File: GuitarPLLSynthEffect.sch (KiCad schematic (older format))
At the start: 26 parts

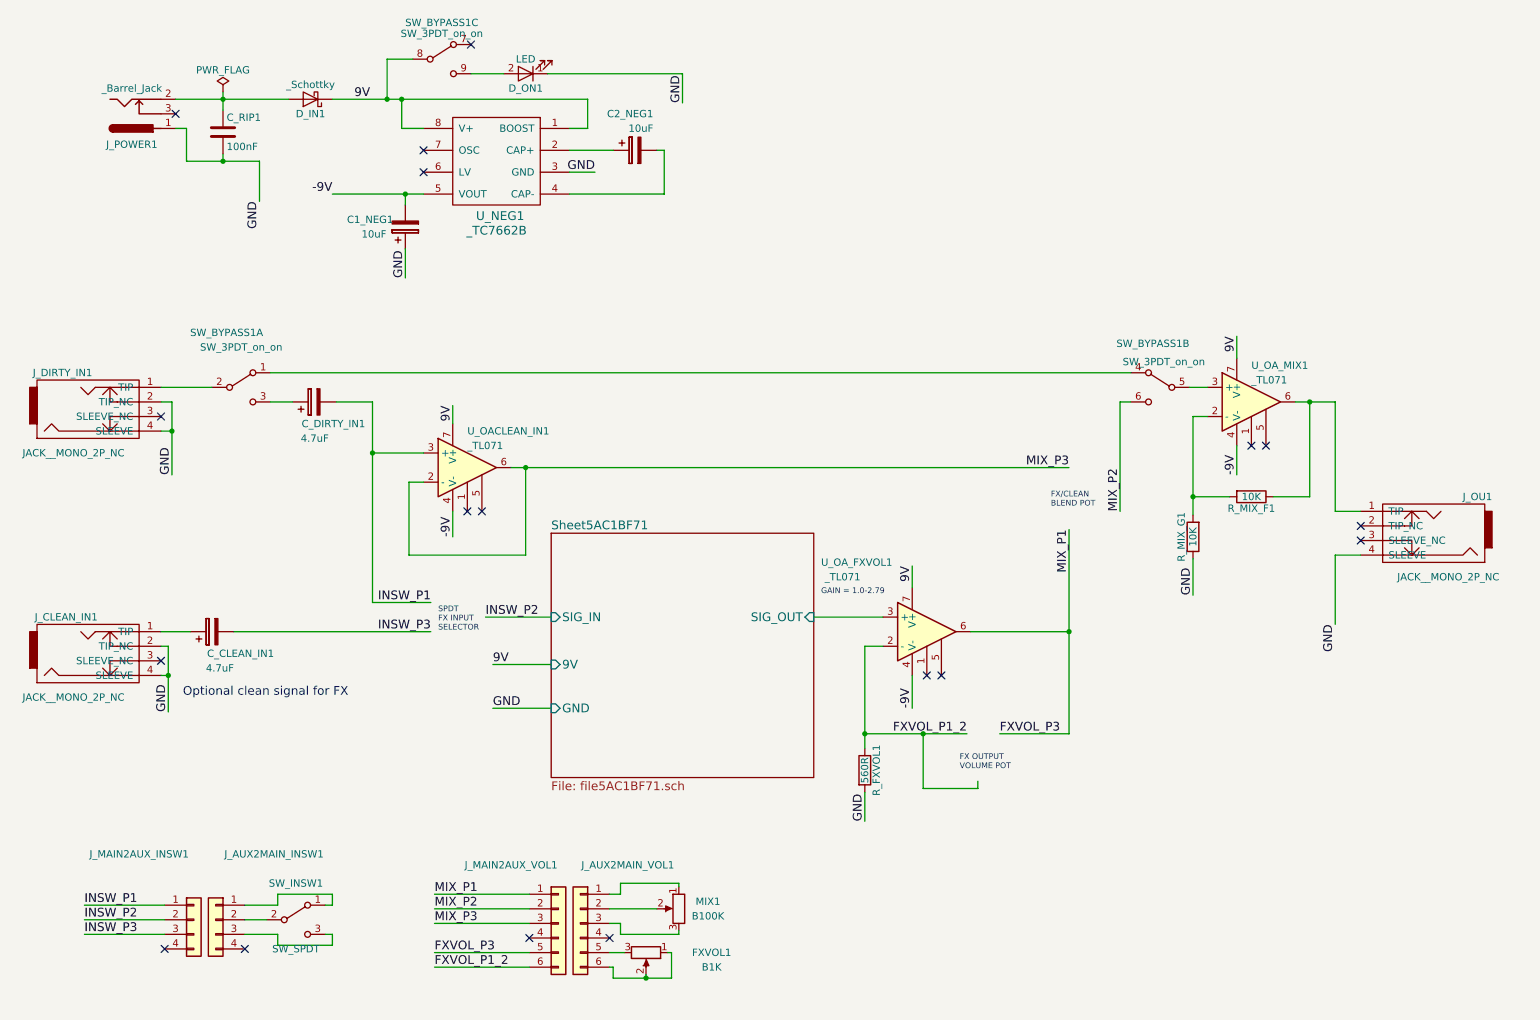
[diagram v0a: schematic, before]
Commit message: Board Design Update RevA
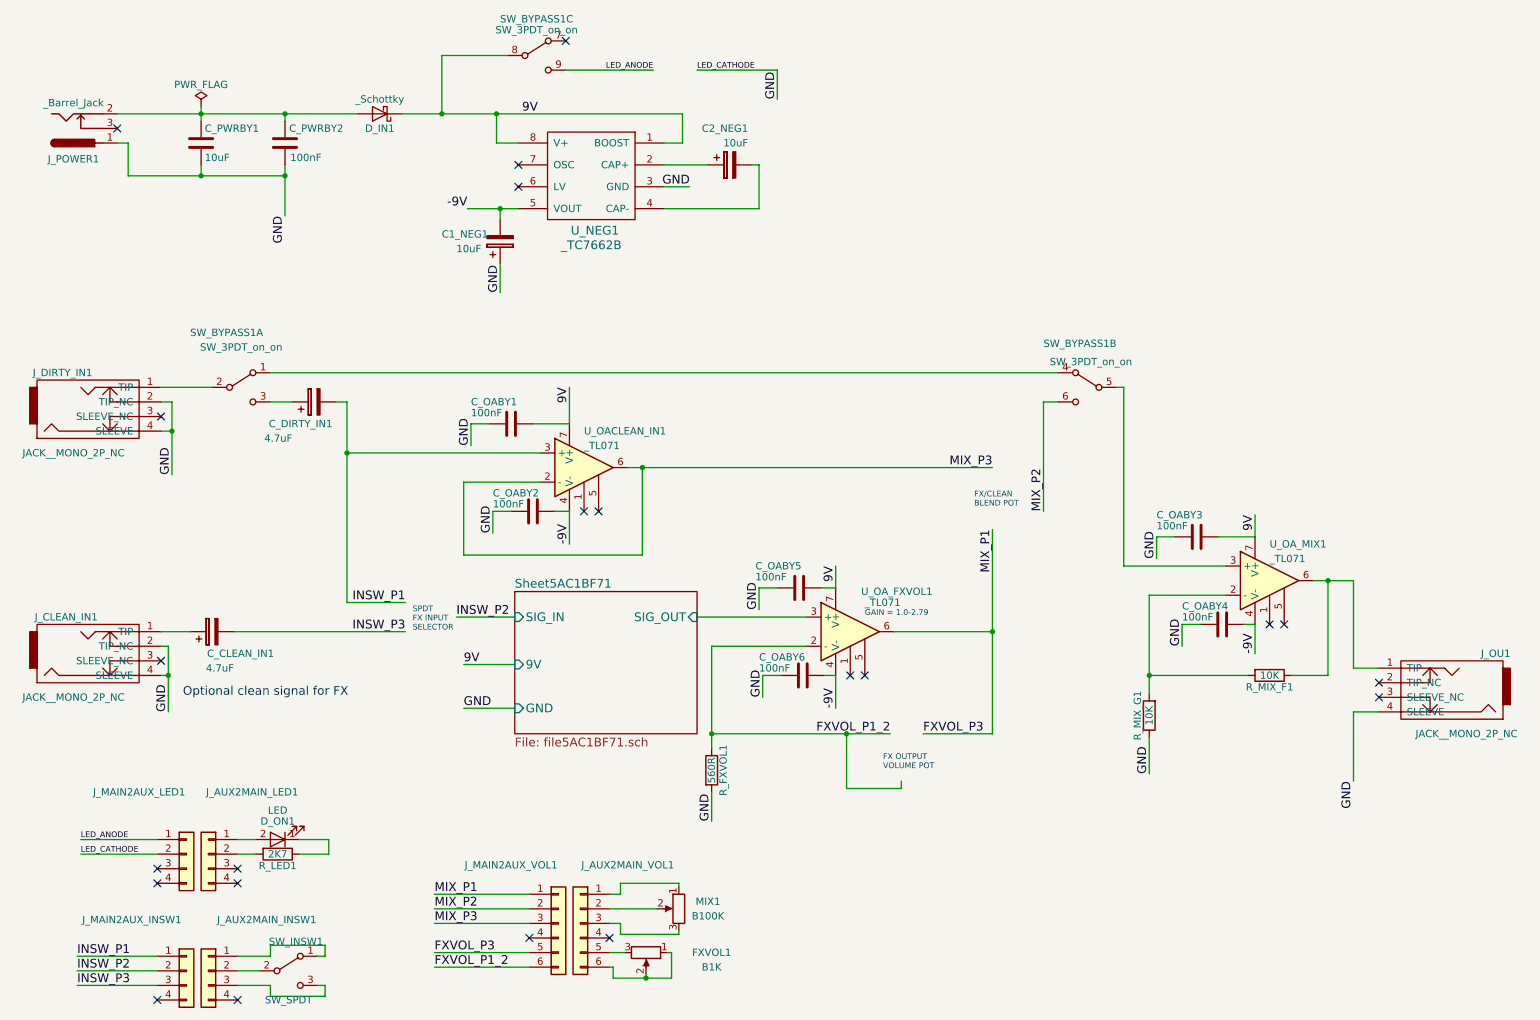
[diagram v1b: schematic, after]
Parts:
- added C_OABY1, C_OABY2, C_OABY3, C_OABY4, C_OABY5, C_OABY6, C_PWRBY2: 100nF, symbol C
- added J_AUX2MAIN_LED1, J_MAIN2AUX_LED1: Conn_01x04, Pin_Headers:Pin_Header_Straight_1x04_Pitch2.54mm, symbol Conn_01x04
- added R_LED1: 2K7, symbol R
- C_PWRBY1: renamed from C_RIP1; value 100nF -> 10uF
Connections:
- net -9V: now also C_OABY2.1, C_OABY4.1, C_OABY6.1
- net 9V: now also C_OABY1.1, C_OABY3.1, C_OABY5.1
- net GND: now also C_OABY1.2, C_OABY2.2, C_OABY3.2, C_OABY4.2, C_OABY5.2, C_OABY6.2, C_PWRBY2.1, J_MAIN2AUX_LED1.2 (Pin_2); no longer D_ON1.1 (K)
- net at C_PWRBY1.1, D_IN1.2 (A), J_POWER1.2: now also C_PWRBY2.2
- net at D_ON1.2 (A): now also J_AUX2MAIN_LED1.1 (Pin_1); no longer SW_BYPASS1.9 (C)
- new net: J_AUX2MAIN_LED1.2 (Pin_2), R_LED1.2
- new net: D_ON1.1 (K), R_LED1.1
- new net LED_ANODE: J_MAIN2AUX_LED1.1 (Pin_1), SW_BYPASS1.9 (C)
- no-connect marks 18 -> 22
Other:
- moved on the sheet: C1_NEG1, C2_NEG1, C_PWRBY1, D_IN1, D_ON1, J_AUX2MAIN_INSW1, J_MAIN2AUX_INSW1, J_OU1, J_POWER1, R_FXVOL1, R_MIX_F1, R_MIX_G1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

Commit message: update
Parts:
- C_OABY1, C_OABY2, C_OABY3, C_OABY4, C_OABY5, C_OABY6, C_PWRBY2: footprint (none) -> Capacitors_SMD:C_0805_HandSoldering
- C_PWRBY1: footprint Capacitors_SMD:CP_Elec_4x5.3 -> Capacitors_SMD:C_0805_HandSoldering
- R_LED1: footprint (none) -> Resistors_SMD:R_0805_HandSoldering
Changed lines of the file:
@@
 F 0 "C_PWRBY1" H 2075 1700 50  0000 L CNN
 F 1 "10uF" H 2075 1500 50  0000 L CNN
-F 2 "Capacitors_SMD:CP_Elec_4x5.3" H 2088 1450 50  0001 C CNN
+F 2 "Capacitors_SMD:C_0805_HandSoldering" H 2088 1450 50  0001 C CNN
 F 3 "" H 2050 1600 50  0001 C CNN
 	1    2050 1600
@@
 F 0 "R_LED1" V 2655 6475 50  0000 C CNN
 F 1 "2K7" V 2575 6475 50  0000 C CNN
-F 2 "" V 2505 6475 50  0001 C CNN
+F 2 "Resistors_SMD:R_0805_HandSoldering" V 2505 6475 50  0001 C CNN
 F 3 "" H 2575 6475 50  0001 C CNN
 	1    2575 6475
@@
 F 0 "C_OABY1" V 4025 3250 50  0000 L CNN
 F 1 "100nF" V 4100 3250 50  0000 L CNN
-F 2 "" H 4213 3375 50  0001 C CNN
+F 2 "Capacitors_SMD:C_0805_HandSoldering" H 4213 3375 50  0001 C CNN
 F 3 "" H 4175 3525 50  0001 C CNN
 	1    4175 3525
@@
 F 0 "C_OABY5" V 6000 4350 50  0000 L CNN
 F 1 "100nF" V 6075 4350 50  0000 L CNN
-F 2 "" H 6188 4500 50  0001 C CNN
+F 2 "Capacitors_SMD:C_0805_HandSoldering" H 6188 4500 50  0001 C CNN
 F 3 "" H 6150 4650 50  0001 C CNN
 	1    6150 4650
@@
 F 0 "C_OABY3" V 8725 4025 50  0000 L CNN
 F 1 "100nF" V 8800 4025 50  0000 L CNN
-F 2 "" H 8913 4150 50  0001 C CNN
+F 2 "Capacitors_SMD:C_0805_HandSoldering" H 8913 4150 50  0001 C CNN
 F 3 "" H 8875 4300 50  0001 C CNN
 	1    8875 4300
@@
 F 0 "C_OABY2" V 4200 3850 50  0000 L CNN
 F 1 "100nF" V 4275 3850 50  0000 L CNN
-F 2 "" H 4363 3975 50  0001 C CNN
+F 2 "Capacitors_SMD:C_0805_HandSoldering" H 4363 3975 50  0001 C CNN
 F 3 "" H 4325 4125 50  0001 C CNN
 	1    4325 4125
@@
 F 0 "C_OABY4" V 8925 4625 50  0000 L CNN
 F 1 "100nF" V 9000 4625 50  0000 L CNN
-F 2 "" H 9088 4750 50  0001 C CNN
+F 2 "Capacitors_SMD:C_0805_HandSoldering" H 9088 4750 50  0001 C CNN
 F 3 "" H 9050 4900 50  0001 C CNN
 	1    9050 4900
@@
 F 0 "C_OABY6" V 6050 4950 50  0000 L CNN
 F 1 "100nF" V 6125 4950 50  0000 L CNN
-F 2 "" H 6213 5100 50  0001 C CNN
+F 2 "Capacitors_SMD:C_0805_HandSoldering" H 6213 5100 50  0001 C CNN
 F 3 "" H 6175 5250 50  0001 C CNN
 	1    6175 5250
@@
 F 0 "C_PWRBY2" H 2225 1500 50  0000 L CNN
 F 1 "100nF" H 2375 1700 50  0000 L CNN
-F 2 "" H 2663 1450 50  0001 C CNN
+F 2 "Capacitors_SMD:C_0805_HandSoldering" H 2663 1450 50  0001 C CNN
 F 3 "" H 2625 1600 50  0001 C CNN
 	1    2625 1600
